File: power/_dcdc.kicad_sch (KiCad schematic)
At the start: 24 parts, among them U5 TPS56A37RPAR

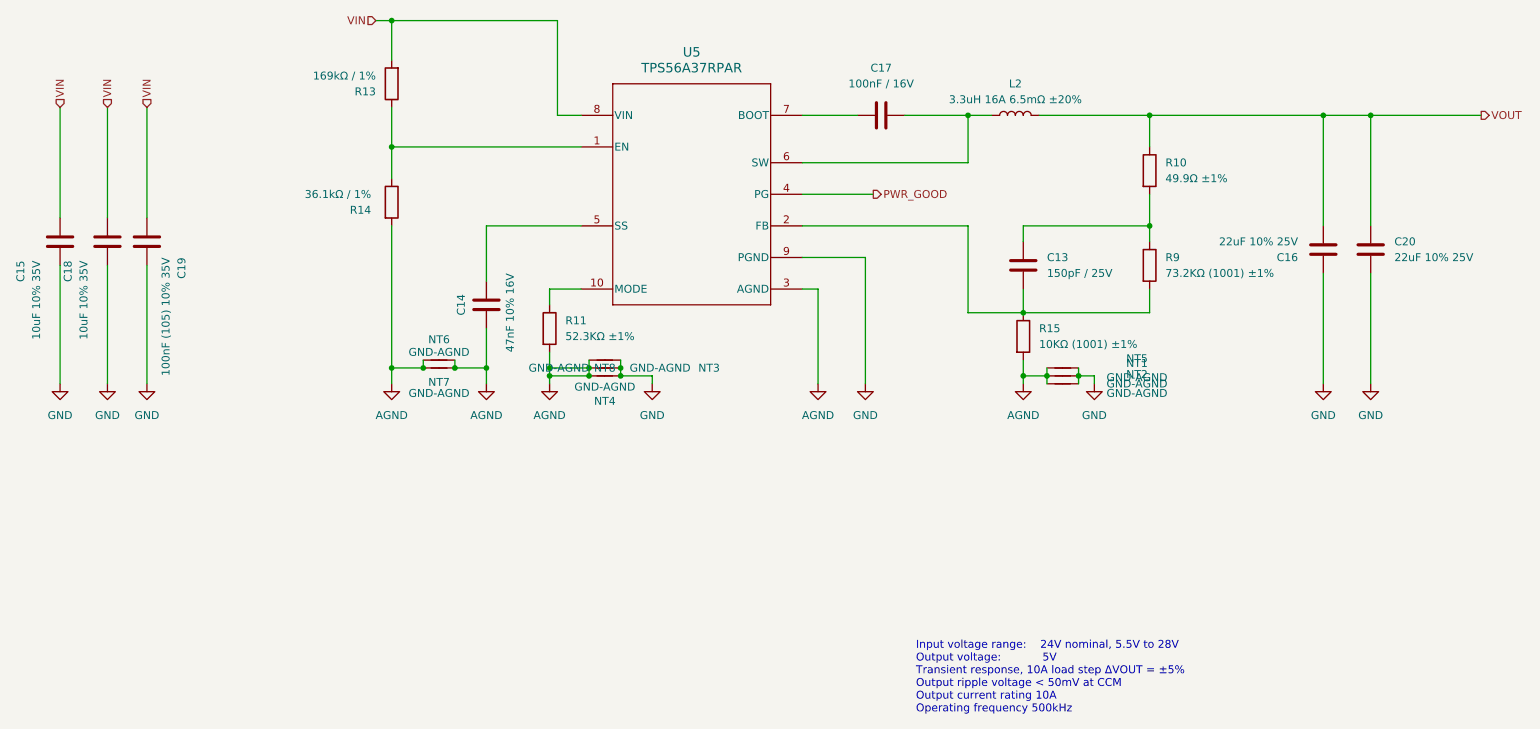
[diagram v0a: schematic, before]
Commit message: preliminary complete layout
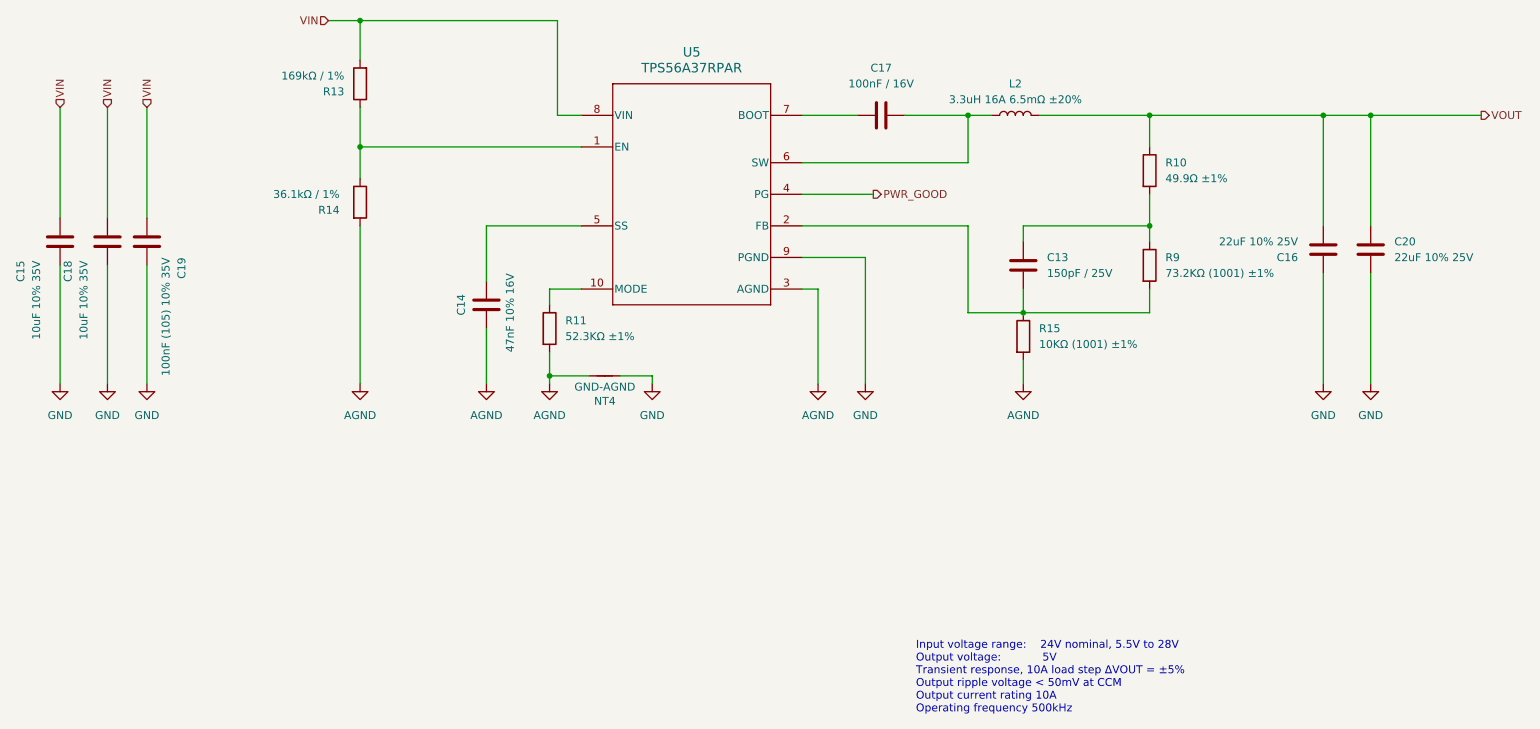
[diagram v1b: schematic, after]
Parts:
- removed NT1, NT2, NT3, NT5, NT6, NT7, NT8: GND-AGND, pilotpi:NetTie-2_THT_Pad0.3mm, symbol Device:NetTie_2
- NT4: footprint pilotpi:NetTie-2_THT_Pad0.3mm -> NetTie:NetTie-2_THT_Pad0.3mm
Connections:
- net AGND: now also NT4.1; no longer NT4.2
- net GND: now also NT4.2; no longer NT4.1
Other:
- moved on the sheet: NT4, R13, R14
